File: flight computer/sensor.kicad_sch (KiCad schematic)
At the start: 92 parts, among them J1 Micro_SD_Card_Det1, J12 Conn_01x04, J13 1x3 servo, J14 1x3 servo, J15 arming terminal, J16 arming terminal, J17 H9161TR-ND, J19 Screw_Terminal_01x02, J20 Screw_Terminal_01x02, J3 H9161TR-ND, J4 H9161TR-ND, J5 Screw_Term, J6 1x3 servo, J9 1x3 servo, Q7 BSS138, Q8 IRLML6402, Q9 IRLML6402, U10 LSM6DS3, U11 BGM220SC12WGA2R, U16 SX1262IMLTRT, U17 PE4259, U5 LPS22HB, U6 GPS, U8 NAND, Y2 32MHz

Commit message: added BGM220SC12WGA2R
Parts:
- J17, J3, J4: footprint U.FL-R-SMT_01_:HRS_U.FL-R-SMT_01_ -> Connector_Coaxial:U.FL_Hirose_U.FL-R-SMT-1_Vertical
- U11: footprint BGM220SC12WGA2R:BGM220SC12WGA2R -> BGM220SC12WGA2R:BGM220S_SIL
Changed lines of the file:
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@@
 			)
 		)
-		(property "Footprint" "U.FL-R-SMT_01_:HRS_U.FL-R-SMT_01_"
+		(property "Footprint" "Connector_Coaxial:U.FL_Hirose_U.FL-R-SMT-1_Vertical"
 			(at 114.3 49.53 0)
 			(effects
@@
 			)
 		)
-		(property "Footprint" "BGM220SC12WGA2R:BGM220SC12WGA2R"
+		(property "Footprint" "BGM220SC12WGA2R:BGM220S_SIL"
 			(at -83.82 81.28 0)
 			(effects
@@
 			)
 		)
-		(property "Footprint" "U.FL-R-SMT_01_:HRS_U.FL-R-SMT_01_"
+		(property "Footprint" "Connector_Coaxial:U.FL_Hirose_U.FL-R-SMT-1_Vertical"
 			(at -7.62 232.41 0)
 			(effects
@@
 			)
 		)
-		(property "Footprint" "U.FL-R-SMT_01_:HRS_U.FL-R-SMT_01_"
+		(property "Footprint" "Connector_Coaxial:U.FL_Hirose_U.FL-R-SMT-1_Vertical"
 			(at -8.89 91.44 0)
 			(effects

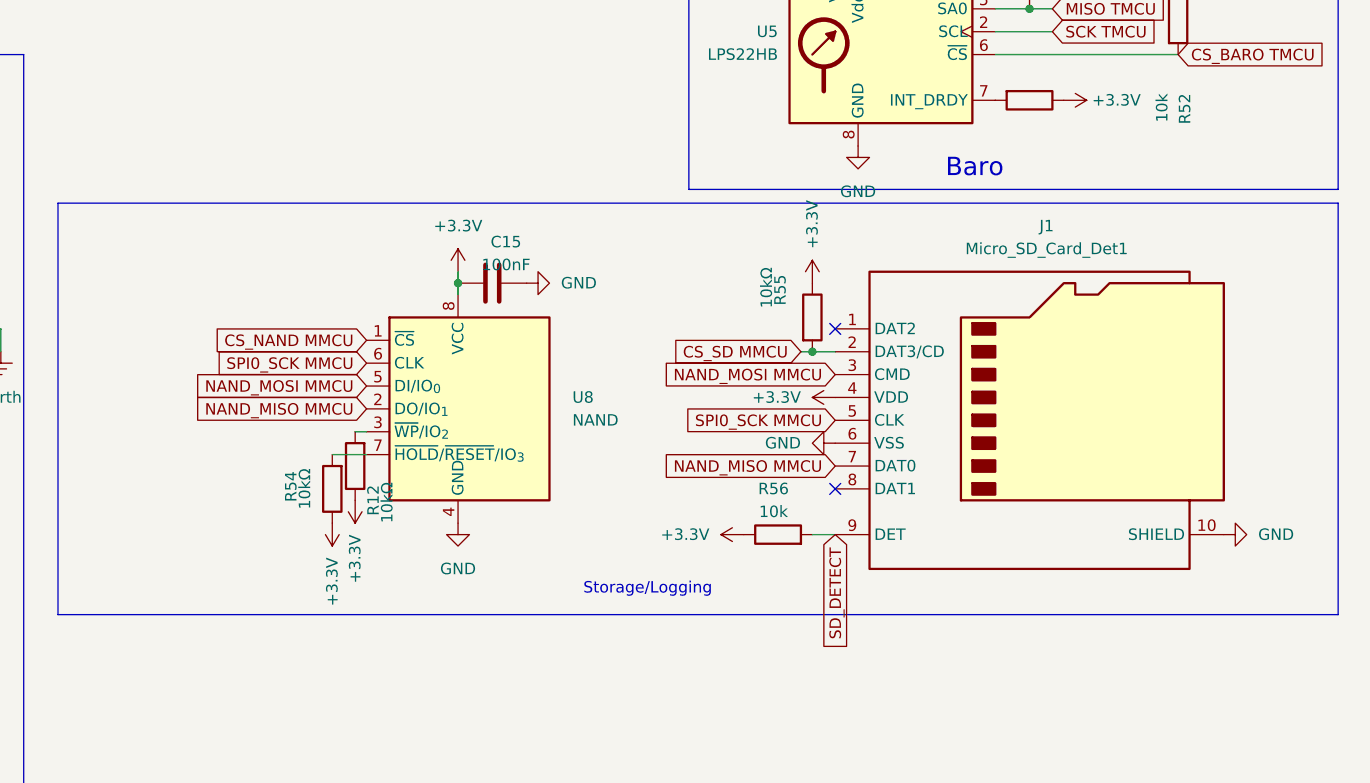
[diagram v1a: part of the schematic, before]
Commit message: force push :'/
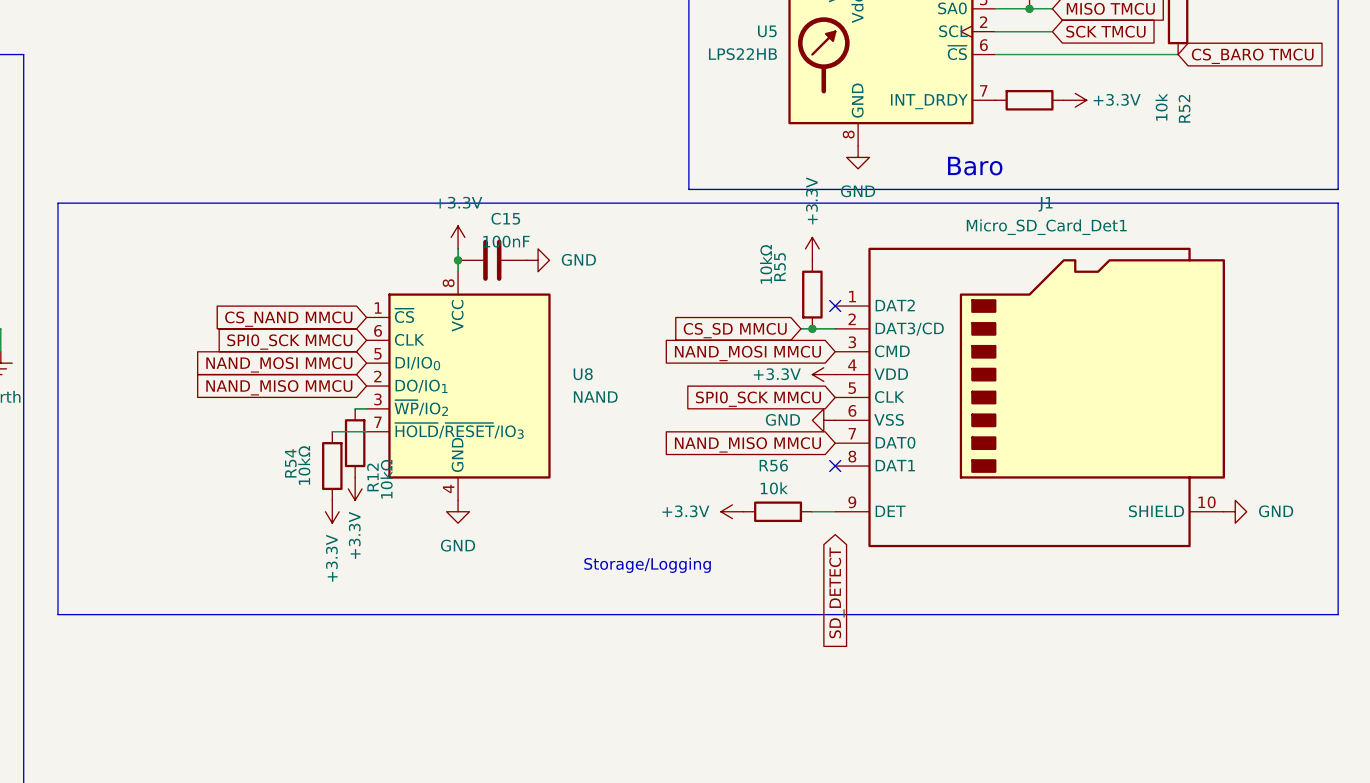
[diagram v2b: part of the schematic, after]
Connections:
- net SD_DETECT: no longer J1.9 (DET), R56.2
- new net: J1.9 (DET), R56.2
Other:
- moved on the sheet: C15, J1, R12, R54, R55, R56, U8

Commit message: added buzzer footprint
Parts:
- BZ2: footprint (none) -> Buzzer:MLT-8530_JHE
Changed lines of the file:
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@@
 			)
 		)
-		(property "Footprint" ""
+		(property "Footprint" "Buzzer:MLT-8530_JHE"
 			(at 35.56 88.9 0)
 			(effects
